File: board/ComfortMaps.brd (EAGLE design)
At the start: 87.6 x 49.6 mm, 47 parts, among them J1 PROG_HDR, J5 0545482271, J6 0545482271, U1 ADXL362, U3 ADP160-3.3, U4 MCP73833, X1 RASPI_GPIO_B+#_PIN

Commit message: Updating board, needs components on digikey.
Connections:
- removed net 5V0A: X1.2
- removed net 5V0B: X1.4
- removed net GND_A: X1.6
- removed net GND_B: X1.9
- removed net GND_C: X1.14
- removed net GND_D: X1.20
- removed net GND_E: X1.25
- removed net GND_F: X1.30
- removed net GND_G: X1.34
- removed net GND_H: X1.39
- new net 3V3A: X1.1
- net GND: now also X1.14, X1.20, X1.25, X1.30, X1.34, X1.39, X1.6, X1.9
- net VOUT: now also X1.2, X1.4; no longer X1.1
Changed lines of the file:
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@@
 <layer number="1" name="Top" color="4" fill="1" visible="yes" active="yes"/>
 <layer number="2" name="Route2" color="1" fill="3" visible="yes" active="yes"/>
-<layer number="15" name="Route15" color="4" fill="6" visible="no" active="yes"/>
+<layer number="15" name="Route15" color="4" fill="6" visible="yes" active="yes"/>
 <layer number="16" name="Bottom" color="1" fill="1" visible="yes" active="yes"/>
 <layer number="17" name="Pads" color="2" fill="1" visible="yes" active="yes"/>
@@
 <contactref element="Q1" pad="5"/>
 <contactref element="JP3" pad="2"/>
-<contactref element="X1" pad="1"/>
-<wire x1="11.43" y1="41.91" x2="70.485" y2="1.905" width="0" layer="19" extent="1-1"/>
+<contactref element="X1" pad="2"/>
+<contactref element="X1" pad="4"/>
+<wire x1="67.945" y1="-0.635" x2="70.485" y2="-0.635" width="0" layer="19" extent="1-1"/>
+<wire x1="11.43" y1="41.91" x2="67.945" y2="-0.635" width="0" layer="19" extent="1-1"/>
 <wire x1="4.862" y1="37.043" x2="11.43" y2="41.91" width="0" layer="19" extent="1-1"/>
 <wire x1="4.862" y1="36.393" x2="4.862" y2="37.043" width="0" layer="19" extent="1-1"/>
@@
 <contactref element="R12" pad="1"/>
 <contactref element="J4" pad="2"/>
+<contactref element="X1" pad="6"/>
+<contactref element="X1" pad="9"/>
+<contactref element="X1" pad="14"/>
+<contactref element="X1" pad="20"/>
+<contactref element="X1" pad="25"/>
+<contactref element="X1" pad="30"/>
+<contactref element="X1" pad="34"/>
+<contactref element="X1" pad="39"/>
 <wire x1="84.735" y1="29.974" x2="84.184" y2="36.306" width="0" layer="19" extent="1-16"/>
 <wire x1="83.82" y1="28.879" x2="84.735" y2="29.974" width="0" layer="19" extent="1-16"/>
@@
 <wire x1="70.17" y1="33.782" x2="70.27" y2="36.576" width="0" layer="19" extent="1-1"/>
 <wire x1="71.97" y1="41.656" x2="70.27" y2="39.116" width="0" layer="19" extent="1-1"/>
-<wire x1="21.424" y1="34.417" x2="70.17" y2="33.782" width="0" layer="19" extent="1-1"/>
+<wire x1="65.405" y1="-0.635" x2="84.735" y2="21.334" width="0" layer="19" extent="1-1"/>
+<wire x1="60.325" y1="1.905" x2="65.405" y2="-0.635" width="0" layer="19" extent="1-1"/>
+<wire x1="55.245" y1="-0.635" x2="60.325" y2="1.905" width="0" layer="19" extent="1-1"/>
+<wire x1="47.625" y1="-0.635" x2="55.245" y2="-0.635" width="0" layer="19" extent="1-1"/>
+<wire x1="40.005" y1="1.905" x2="47.625" y2="-0.635" width="0" layer="19" extent="1-1"/>
+<wire x1="34.925" y1="-0.635" x2="40.005" y2="1.905" width="0" layer="19" extent="1-1"/>
+<wire x1="29.845" y1="-0.635" x2="34.925" y2="-0.635" width="0" layer="19" extent="1-1"/>
+<wire x1="22.225" y1="1.905" x2="29.845" y2="-0.635" width="0" layer="19" extent="1-1"/>
+<wire x1="18.415" y1="6.938" x2="22.225" y2="1.905" width="0" layer="19" extent="1-1"/>
+<wire x1="19.304" y1="-4.318" x2="22.225" y2="1.905" width="0" layer="19" extent="1-1"/>
+<wire x1="7.112" y1="-4.064" x2="19.304" y2="-4.318" width="0" layer="19" extent="1-1"/>
+<wire x1="6.604" y1="25.742" x2="18.415" y2="6.938" width="0" layer="19" extent="1-1"/>
+<wire x1="5.456" y1="29.218" x2="6.604" y2="25.742" width="0" layer="19" extent="1-1"/>
+<wire x1="5.858" y1="31.1442" x2="5.456" y2="29.218" width="0" layer="19" extent="1-1"/>
+<wire x1="6.358" y1="31.1442" x2="5.858" y2="31.1442" width="0" layer="19" extent="1-1"/>
+<wire x1="9.362" y1="35.093" x2="6.358" y2="31.1442" width="0" layer="19" extent="1-1"/>
+<wire x1="13.55" y1="33.782" x2="9.362" y2="35.093" width="0" layer="19" extent="1-1"/>
+<wire x1="16.51" y1="34.1329" x2="13.55" y2="33.782" width="0" layer="19" extent="1-1"/>
+<wire x1="16.637" y1="29.884" x2="16.51" y2="34.1329" width="0" layer="19" extent="1-1"/>
+<wire x1="21.424" y1="34.417" x2="16.51" y2="34.1329" width="0" layer="19" extent="1-1"/>
 <wire x1="21.424" y1="36.83" x2="21.424" y2="34.417" width="0" layer="19" extent="1-1"/>
-<wire x1="16.51" y1="34.1329" x2="21.424" y2="34.417" width="0" layer="19" extent="1-1"/>
-<wire x1="13.55" y1="33.782" x2="16.51" y2="34.1329" width="0" layer="19" extent="1-1"/>
-<wire x1="16.637" y1="29.884" x2="16.51" y2="34.1329" width="0" layer="19" extent="1-1"/>
-<wire x1="9.362" y1="35.093" x2="13.55" y2="33.782" width="0" layer="19" extent="1-1"/>
-<wire x1="6.358" y1="31.1442" x2="9.362" y2="35.093" width="0" layer="19" extent="1-1"/>
-<wire x1="5.858" y1="31.1442" x2="6.358" y2="31.1442" width="0" layer="19" extent="1-1"/>
-<wire x1="5.456" y1="29.218" x2="5.858" y2="31.1442" width="0" layer="19" extent="1-1"/>
-<wire x1="6.604" y1="25.742" x2="5.456" y2="29.218" width="0" layer="19" extent="1-1"/>
 <wire x1="17.78" y1="41.91" x2="21.424" y2="36.83" width="0" layer="19" extent="1-1"/>
 <wire x1="8.89" y1="41.91" x2="9.362" y2="35.093" width="0" layer="19" extent="1-1"/>
-<wire x1="18.415" y1="6.938" x2="6.604" y2="25.742" width="0" layer="19" extent="1-1"/>
-<wire x1="19.304" y1="-4.318" x2="18.415" y2="6.938" width="0" layer="19" extent="1-1"/>
-<wire x1="7.112" y1="-4.064" x2="19.304" y2="-4.318" width="0" layer="19" extent="1-1"/>
 </signal>
 <signal name="OVERRIDE">
@@
 <wire x1="15.875" y1="6.938" x2="23.052" y2="31.496" width="0" layer="19" extent="1-1"/>
 </signal>
-<signal name="5V0A">
-<contactref element="X1" pad="2"/>
-</signal>
-<signal name="GND_A">
-<contactref element="X1" pad="6"/>
-</signal>
-<signal name="5V0B">
-<contactref element="X1" pad="4"/>
-</signal>
 <signal name="3V3B">
 <contactref element="X1" pad="17"/>
-</signal>
-<signal name="GND_B">
-<contactref element="X1" pad="9"/>
-</signal>
-<signal name="GND_C">
-<contactref element="X1" pad="14"/>
-</signal>
-<signal name="GND_D">
-<contactref element="X1" pad="20"/>
-</signal>
-<signal name="GND_E">
-<contactref element="X1" pad="25"/>
-</signal>
-<signal name="GND_F">
-<contactref element="X1" pad="30"/>
-</signal>
-<signal name="GND_G">
-<contactref element="X1" pad="34"/>
-</signal>
-<signal name="GND_H">
-<contactref element="X1" pad="39"/>
 </signal>
 <signal name="GPIO17">
@@
 <wire x1="44.24" y1="37.32" x2="85.58" y2="7.83" width="0" layer="19" extent="1-1"/>
 </signal>
+<signal name="3V3A">
+<contactref element="X1" pad="1"/>
+</signal>
 </signals>

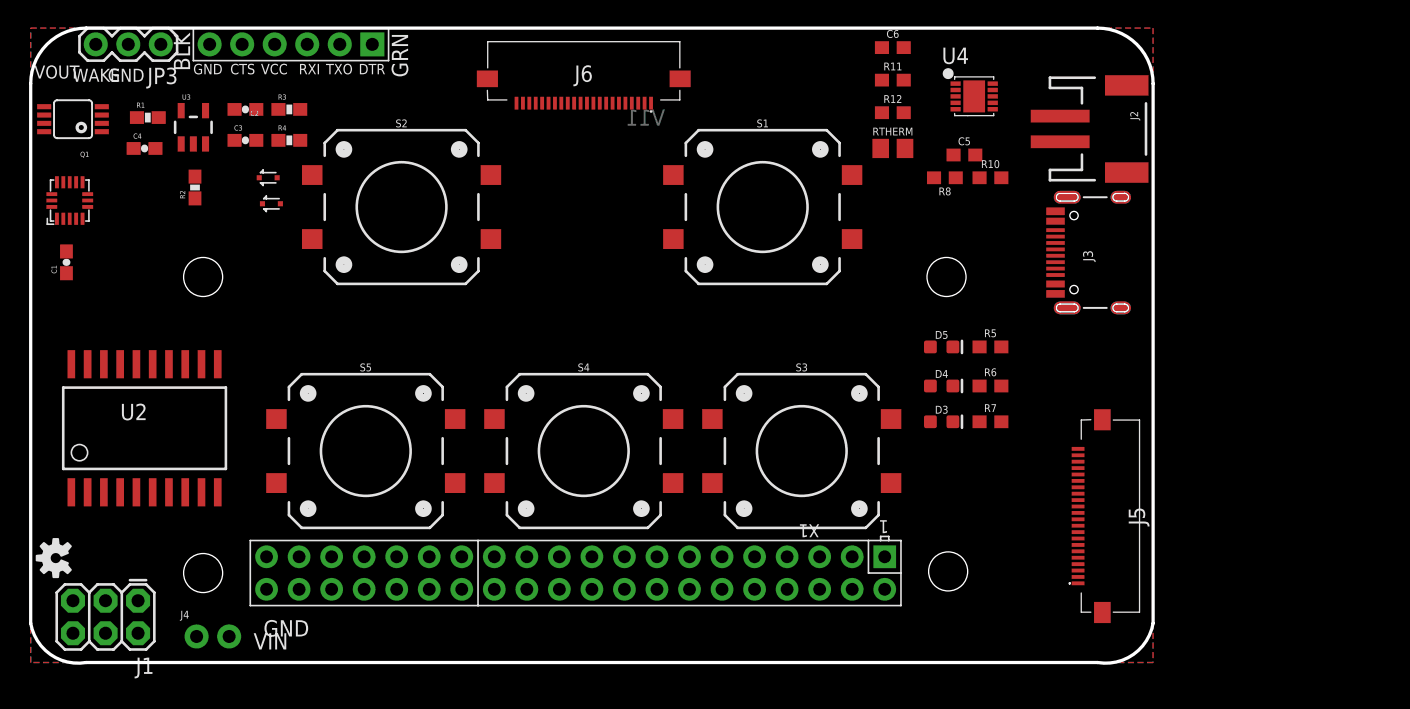
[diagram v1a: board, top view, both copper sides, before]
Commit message: Triangle board.
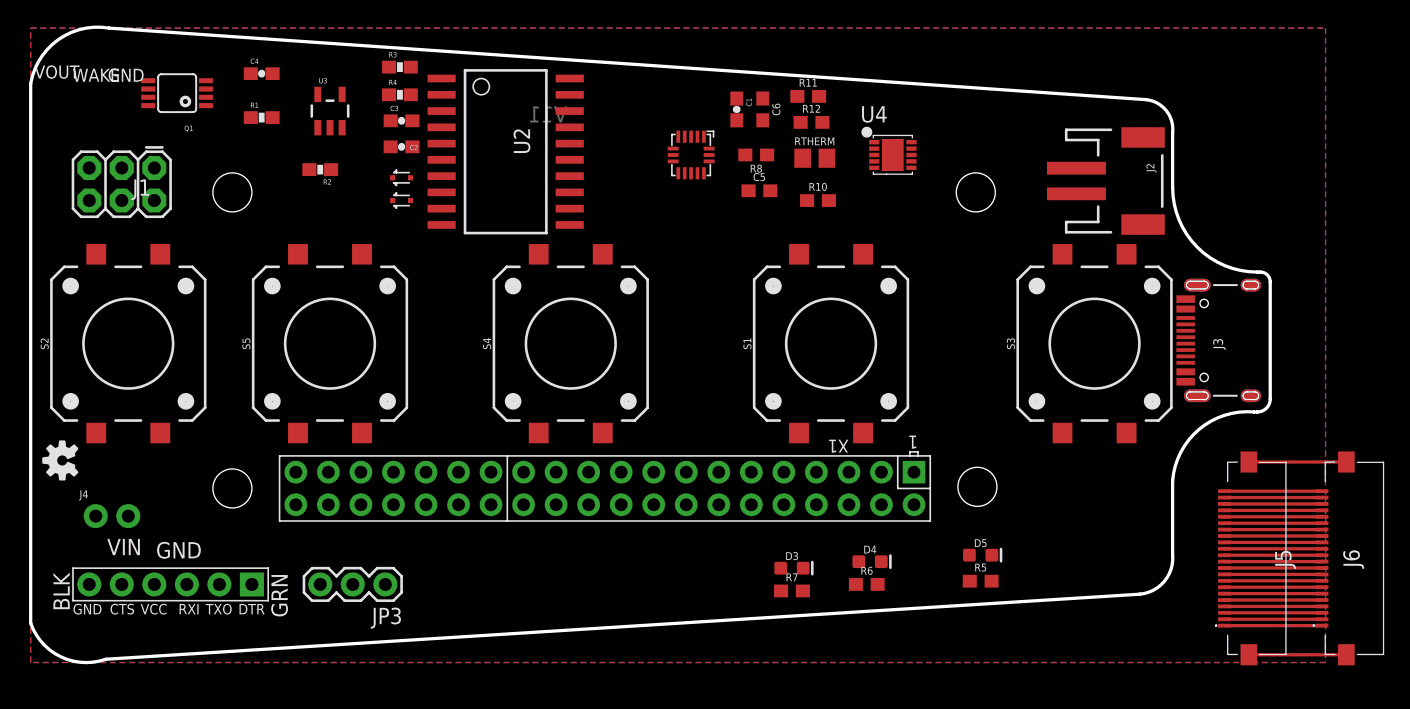
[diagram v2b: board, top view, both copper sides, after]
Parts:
- moved J6 70.5 mm to (106.7, 1.78), turned to 90 degrees
- moved C1 53.7 mm to (58.9, 36.8), turned to 270 degrees
- moved U1 48.6 mm to (55.4, 33.3), turned to 270 degrees
- moved JP3 45.7 mm to (31.5, -0.25)
- moved JP1 43.2 mm to (14.7, -0.25)
- moved U2 35.5 mm to (40.9, 33.5), turned to 270 degrees
- moved J1 33.8 mm to (13.5, 32.3)
- moved S3 24.3 mm to (86.9, 18.5), turned to 90 degrees
- moved S2 23.9 mm to (11.4, 18.5), turned to 90 degrees
- moved R7 20.4 mm to (63.2, -0.76)
- moved R5 18.3 mm to (78.0, 0.00)
- moved R6 18.3 mm to (69.1, -0.25)
- moved D5 16.5 mm to (78.0, 2.03)
- moved D3 16.3 mm to (63.2, 1.02)
- moved C5 16.2 mm to (60.7, 30.5)
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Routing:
- net CSI24: track 0.00 -> 7.62 mm
- net CSI23: track 0.00 -> 7.62 mm
- net CSI9: track 0.00 -> 7.62 mm
- net CSI8: track 0.00 -> 7.62 mm
- net CSI7: track 0.00 -> 7.62 mm
- net CSI6: track 0.00 -> 7.62 mm
- net CSI5: track 0.00 -> 7.62 mm
- net CSI4: track 0.00 -> 7.62 mm
- net CSI3: track 0.00 -> 7.62 mm
- net CSI22: track 0.00 -> 7.62 mm
- net CSI21: track 0.00 -> 7.62 mm
- net CSI20: track 0.00 -> 7.62 mm
- net CSI2: track 0.00 -> 7.62 mm
- net CSI19: track 0.00 -> 7.62 mm
- net CSI18: track 0.00 -> 7.62 mm
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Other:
- board size 87.6 x 49.6 mm -> 96.8 x 49.6 mm
